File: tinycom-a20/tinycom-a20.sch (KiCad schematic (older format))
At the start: 36 parts, among them P1 CONN_02X08, P2 CONN_02X08, U1 ALLWINNERA10/TFBGA441, U2 H5TQG63BFR/FBGA96, U3 H27UBG8T2A/TSOP48, Y1 Crystal_Small, Y2 Crystal_Small

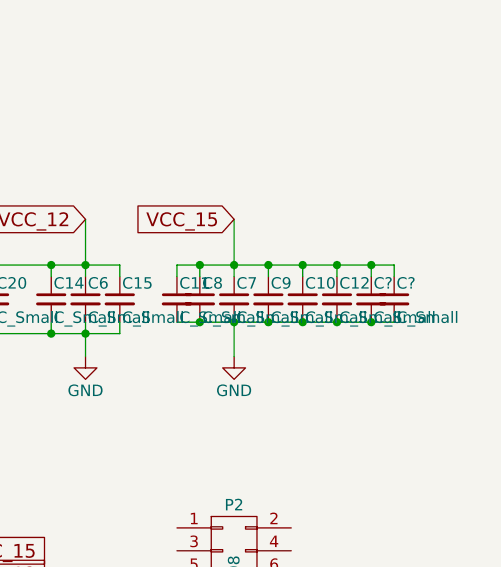
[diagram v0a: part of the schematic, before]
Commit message: add power routes
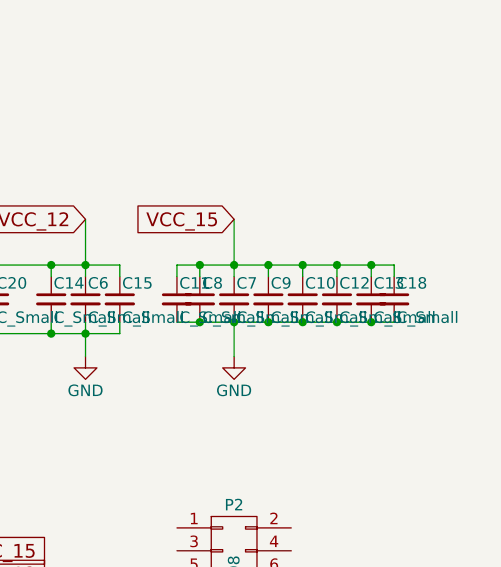
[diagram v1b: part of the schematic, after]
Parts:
- gave numbers to parts that had none: 2
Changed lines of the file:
@@
 $EndComp
 $Comp
-L GND #PWR01
+L GND #PWR21
 U 1 1 563E445F
 P 17800 6150
-F 0 "#PWR01" H 17800 5900 50  0001 C CNN
+F 0 "#PWR21" H 17800 5900 50  0001 C CNN
 F 1 "GND" H 17800 6000 50  0000 C CNN
 F 2 "" H 17800 6150 60  0000 C CNN
@@
 SCK_P
 $Comp
-L GND #PWR02
+L GND #PWR19
 U 1 1 563ECE56
 P 14950 850
-F 0 "#PWR02" H 14950 600 50  0001 C CNN
+F 0 "#PWR19" H 14950 600 50  0001 C CNN
 F 1 "GND" H 14950 700 50  0000 C CNN
 F 2 "" H 14950 850 60  0000 C CNN
@@
 $EndComp
 $Comp
-L GND #PWR03
+L GND #PWR17
 U 1 1 563EDF36
 P 13600 5900
-F 0 "#PWR03" H 13600 5650 50  0001 C CNN
+F 0 "#PWR17" H 13600 5650 50  0001 C CNN
 F 1 "GND" H 13600 5750 50  0000 C CNN
 F 2 "" H 13600 5900 60  0000 C CNN
@@
 $EndComp
 $Comp
-L GND #PWR04
+L GND #PWR18
 U 1 1 563EE398
 P 14350 5150
-F 0 "#PWR04" H 14350 4900 50  0001 C CNN
+F 0 "#PWR18" H 14350 4900 50  0001 C CNN
 F 1 "GND" H 14350 5000 50  0000 C CNN
 F 2 "" H 14350 5150 60  0000 C CNN
@@
 $EndComp
 $Comp
-L GND #PWR05
+L GND #PWR10
 U 1 1 56400687
 P 12400 9950
-F 0 "#PWR05" H 12400 9700 50  0001 C CNN
+F 0 "#PWR10" H 12400 9700 50  0001 C CNN
 F 1 "GND" H 12400 9800 50  0000 C CNN
 F 2 "" H 12400 9950 60  0000 C CNN
@@
 $EndComp
 $Comp
-L GND #PWR06
+L GND #PWR11
 U 1 1 56400704
 P 12650 9950
-F 0 "#PWR06" H 12650 9700 50  0001 C CNN
+F 0 "#PWR11" H 12650 9700 50  0001 C CNN
 F 1 "GND" H 12650 9800 50  0000 C CNN
 F 2 "" H 12650 9950 60  0000 C CNN
@@
 $EndComp
 $Comp
-L GND #PWR07
+L GND #PWR9
 U 1 1 56408532
 P 12150 9250
-F 0 "#PWR07" H 12150 9000 50  0001 C CNN
+F 0 "#PWR9" H 12150 9000 50  0001 C CNN
 F 1 "GND" H 12150 9100 50  0000 C CNN
 F 2 "" H 12150 9250 60  0000 C CNN
@@
 $EndComp
 $Comp
-L GND #PWR08
+L GND #PWR12
 U 1 1 56408573
 P 12700 9300
-F 0 "#PWR08" H 12700 9050 50  0001 C CNN
+F 0 "#PWR12" H 12700 9050 50  0001 C CNN
 F 1 "GND" H 12700 9150 50  0000 C CNN
 F 2 "" H 12700 9300 60  0000 C CNN
@@
 $EndComp
 $Comp
-L GND #PWR09
+L GND #PWR14
 U 1 1 5640D8CA
 P 12750 6950
-F 0 "#PWR09" H 12750 6700 50  0001 C CNN
+F 0 "#PWR14" H 12750 6700 50  0001 C CNN
 F 1 "GND" H 12750 6800 50  0000 C CNN
 F 2 "" H 12750 6950 60  0000 C CNN
@@
 $EndComp
 $Comp
-L GND #PWR010
+L GND #PWR24
 U 1 1 56408FCA
 P 19800 9350
-F 0 "#PWR010" H 19800 9100 50  0001 C CNN
+F 0 "#PWR24" H 19800 9100 50  0001 C CNN
 F 1 "GND" H 19800 9200 50  0000 C CNN
 F 2 "" H 19800 9350 60  0000 C CNN
@@
 UDP2
 $Comp
-L GND #PWR011
+L GND #PWR26
 U 1 1 56411561
 P 20650 10200
-F 0 "#PWR011" H 20650 9950 50  0001 C CNN
+F 0 "#PWR26" H 20650 9950 50  0001 C CNN
 F 1 "GND" H 20650 10050 50  0000 C CNN
 F 2 "" H 20650 10200 60  0000 C CNN
@@
 NoConn ~ 7500 2750
 $Comp
-L GND #PWR012
+L GND #PWR8
 U 1 1 56414A5D
 P 8850 1300
-F 0 "#PWR012" H 8850 1050 50  0001 C CNN
+F 0 "#PWR8" H 8850 1050 50  0001 C CNN
 F 1 "GND" H 8850 1150 50  0000 C CNN
 F 2 "" H 8850 1300 60  0000 C CNN
@@
 VCC_15
 $Comp
-L GND #PWR013
+L GND #PWR1
 U 1 1 56417328
 P 800 9350
-F 0 "#PWR013" H 800 9100 50  0001 C CNN
+F 0 "#PWR1" H 800 9100 50  0001 C CNN
 F 1 "GND" H 800 9200 50  0000 C CNN
 F 2 "" H 800 9350 60  0000 C CNN
@@
 NoConn ~ 1050 13300
 $Comp
-L GND #PWR014
+L GND #PWR3
 U 1 1 56417B02
 P 900 13450
-F 0 "#PWR014" H 900 13200 50  0001 C CNN
+F 0 "#PWR3" H 900 13200 50  0001 C CNN
 F 1 "GND" H 900 13300 50  0000 C CNN
 F 2 "" H 900 13450 60  0000 C CNN
@@
 NoConn ~ 1050 13700
 $Comp
-L GND #PWR015
+L GND #PWR2
 U 1 1 56417F5A
 P 850 13800
-F 0 "#PWR015" H 850 13550 50  0001 C CNN
+F 0 "#PWR2" H 850 13550 50  0001 C CNN
 F 1 "GND" H 850 13650 50  0000 C CNN
 F 2 "" H 850 13800 60  0000 C CNN
@@
 NoConn ~ 5650 11400
 $Comp
-L GND #PWR016
+L GND #PWR6
 U 1 1 56418E41
 P 5850 12050
-F 0 "#PWR016" H 5850 11800 50  0001 C CNN
+F 0 "#PWR6" H 5850 11800 50  0001 C CNN
 F 1 "GND" H 5850 11900 50  0000 C CNN
 F 2 "" H 5850 12050 60  0000 C CNN
@@
 $EndComp
 $Comp
-L GND #PWR017
+L GND #PWR7
 U 1 1 56419222
 P 5900 12300
-F 0 "#PWR017" H 5900 12050 50  0001 C CNN
+F 0 "#PWR7" H 5900 12050 50  0001 C CNN
 F 1 "GND" H 5900 12150 50  0000 C CNN
 F 2 "" H 5900 12300 60  0000 C CNN
@@
 NoConn ~ 11650 14450
 $Comp
-L GND #PWR018
+L GND #PWR16
 U 1 1 5641B53D
 P 12900 9850
-F 0 "#PWR018" H 12900 9600 50  0001 C CNN
+F 0 "#PWR16" H 12900 9600 50  0001 C CNN
 F 1 "GND" H 12900 9700 50  0000 C CNN
 F 2 "" H 12900 9850 60  0000 C CNN
@@
 NoConn ~ 13000 10700
 $Comp
-L GND #PWR019
+L GND #PWR15
 U 1 1 5641BA06
 P 12850 11350
-F 0 "#PWR019" H 12850 11100 50  0001 C CNN
+F 0 "#PWR15" H 12850 11100 50  0001 C CNN
 F 1 "GND" H 12850 11200 50  0000 C CNN
 F 2 "" H 12850 11350 60  0000 C CNN
@@
 NoConn ~ 13000 12600
 $Comp
-L GND #PWR020
+L GND #PWR13
 U 1 1 5641C0BF
 P 12700 12700
-F 0 "#PWR020" H 12700 12450 50  0001 C CNN
+F 0 "#PWR13" H 12700 12450 50  0001 C CNN
 F 1 "GND" H 12700 12550 50  0000 C CNN
 F 2 "" H 12700 12700 60  0000 C CNN
@@
 $EndComp
 $Comp
-L GND #PWR021
+L GND #PWR20
 U 1 1 5641C64B
 P 17750 14500
-F 0 "#PWR021" H 17750 14250 50  0001 C CNN
+F 0 "#PWR20" H 17750 14250 50  0001 C CNN
 F 1 "GND" H 17750 14350 50  0000 C CNN
 F 2 "" H 17750 14500 60  0000 C CNN
@@
 $EndComp
 $Comp
-L GND #PWR022
+L GND #PWR22
 U 1 1 5641CC6D
 P 17800 13850
-F 0 "#PWR022" H 17800 13600 50  0001 C CNN
+F 0 "#PWR22" H 17800 13600 50  0001 C CNN
 F 1 "GND" H 17800 13700 50  0000 C CNN
 F 2 "" H 17800 13850 60  0000 C CNN
@@
 VCC_33
 $Comp
-L GND #PWR023
+L GND #PWR27
 U 1 1 5643044F
 P 20800 13600
-F 0 "#PWR023" H 20800 13350 50  0001 C CNN
+F 0 "#PWR27" H 20800 13350 50  0001 C CNN
 F 1 "GND" H 20800 13450 50  0000 C CNN
 F 2 "" H 20800 13600 60  0000 C CNN
@@
 VCC_33
 $Comp
-L GND #PWR024
+L GND #PWR5
 U 1 1 5643A4FE
 P 5850 10900
-F 0 "#PWR024" H 5850 10650 50  0001 C CNN
+F 0 "#PWR5" H 5850 10650 50  0001 C CNN
 F 1 "GND" H 5850 10750 50  0000 C CNN
 F 2 "" H 5850 10900 60  0000 C CNN
@@
 NoConn ~ 1050 14100
 $Comp
-L GND #PWR025
+L GND #PWR4
 U 1 1 5643BDD7
 P 950 11000
-F 0 "#PWR025" H 950 10750 50  0001 C CNN
+F 0 "#PWR4" H 950 10750 50  0001 C CNN
 F 1 "GND" H 950 10850 50  0000 C CNN
 F 2 "" H 950 11000 60  0000 C CNN
@@
 VCC_33
 $Comp
-L GND #PWR026
+L GND #PWR23
 U 1 1 56440C85
 P 19500 8700
-F 0 "#PWR026" H 19500 8450 50  0001 C CNN
+F 0 "#PWR23" H 19500 8450 50  0001 C CNN
 F 1 "GND" H 19500 8550 50  0000 C CNN
 F 2 "" H 19500 8700 60  0000 C CNN
@@
 $EndComp
 $Comp
-L GND #PWR027
+L GND #PWR25
 U 1 1 56441E51
 P 20300 8700
-F 0 "#PWR027" H 20300 8450 50  0001 C CNN
+F 0 "#PWR25" H 20300 8450 50  0001 C CNN
 F 1 "GND" H 20300 8550 50  0000 C CNN
 F 2 "" H 20300 8700 60  0000 C CNN
@@
 $EndComp
 $Comp
-L GND #PWR028
+L GND #PWR28
 U 1 1 564426D1
 P 20950 8700
-F 0 "#PWR028" H 20950 8450 50  0001 C CNN
+F 0 "#PWR28" H 20950 8450 50  0001 C CNN
 F 1 "GND" H 20950 8550 50  0000 C CNN
 F 2 "" H 20950 8700 60  0000 C CNN
@@
 $EndComp
 $Comp
-L C_Small C?
+L C_Small C13
 U 1 1 5645F6BF
 P 21550 8450
-F 0 "C?" H 21560 8520 50  0000 L CNN
+F 0 "C13" H 21560 8520 50  0000 L CNN
 F 1 "C_Small" H 21560 8370 50  0000 L CNN
 F 2 "Capacitors_SMD:C_0603" H 21550 8450 60  0001 C CNN
@@
 $EndComp
 $Comp
-L C_Small C?
+L C_Small C18
 U 1 1 5645F746
 P 21650 8450
-F 0 "C?" H 21660 8520 50  0000 L CNN
+F 0 "C18" H 21660 8520 50  0000 L CNN
 F 1 "C_Small" H 21660 8370 50  0000 L CNN
 F 2 "Capacitors_SMD:C_0603" H 21650 8450 60  0001 C CNN

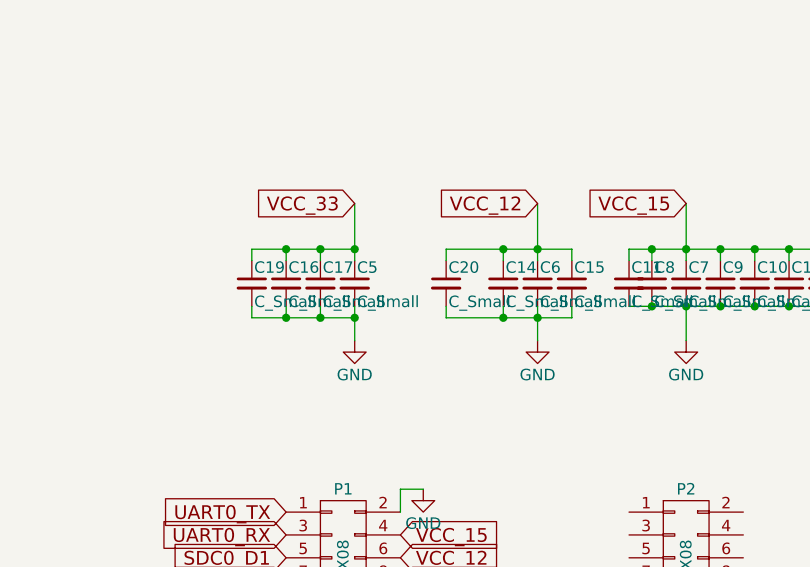
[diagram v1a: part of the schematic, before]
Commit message: fix
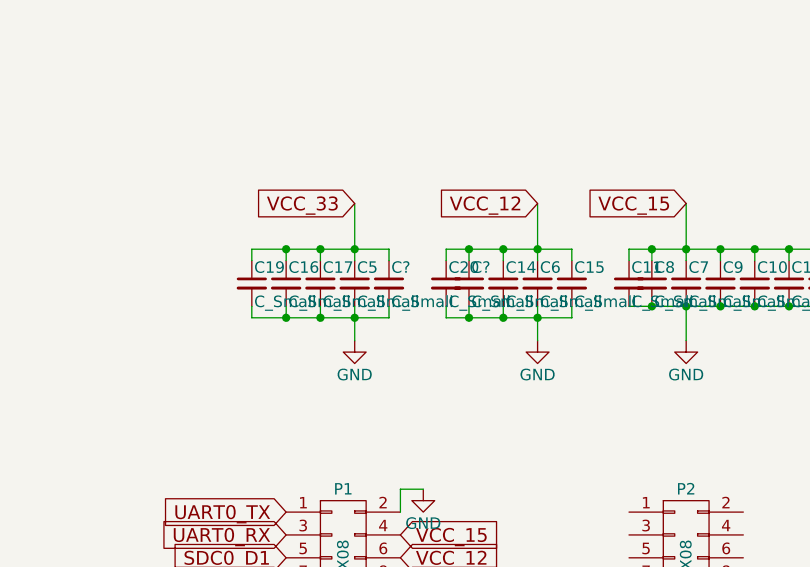
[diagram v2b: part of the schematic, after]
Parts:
- added C? (x2): C_Small, Capacitors_SMD:C_0603, symbol C_Small
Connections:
- net GND: now also C?.2, C?.2
- net VCC_12: now also C?.1
- net VCC_33: now also C?.1
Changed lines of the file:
@@
 	19900 8600 19900 8550
 Wire Wire Line
-	19050 8300 19500 8300
+	19050 8300 19650 8300
 Wire Wire Line
-	19050 8600 19500 8600
+	19050 8600 19650 8600
 Wire Wire Line
 	20700 8550 21650 8550
@@
 Connection ~ 21400 8550
 Connection ~ 21550 8550
+$Comp
+L C_Small C?
+U 1 1 5647248A
+P 20000 8450
+F 0 "C?" H 20010 8520 50  0000 L CNN
+F 1 "C_Small" H 20010 8370 50  0000 L CNN
+F 2 "Capacitors_SMD:C_0603" H 20000 8450 60  0001 C CNN
+F 3 "" H 20000 8450 60  0000 C CNN
+	1    20000 8450
+	1    0    0    -1
+$EndComp
+Wire Wire Line
+	20000 8350 20000 8300
+Connection ~ 20000 8300
+Wire Wire Line
+	20000 8550 20000 8600
+Connection ~ 20000 8600
+$Comp
+L C_Small C?
+U 1 1 56472991
+P 19650 8450
+F 0 "C?" H 19660 8520 50  0000 L CNN
+F 1 "C_Small" H 19660 8370 50  0000 L CNN
+F 2 "Capacitors_SMD:C_0603" H 19650 8450 60  0001 C CNN
+F 3 "" H 19650 8450 60  0000 C CNN
+	1    19650 8450
+	1    0    0    -1
+$EndComp
+Wire Wire Line
+	19650 8300 19650 8350
+Wire Wire Line
+	19650 8600 19650 8550
 $EndSCHEMATC

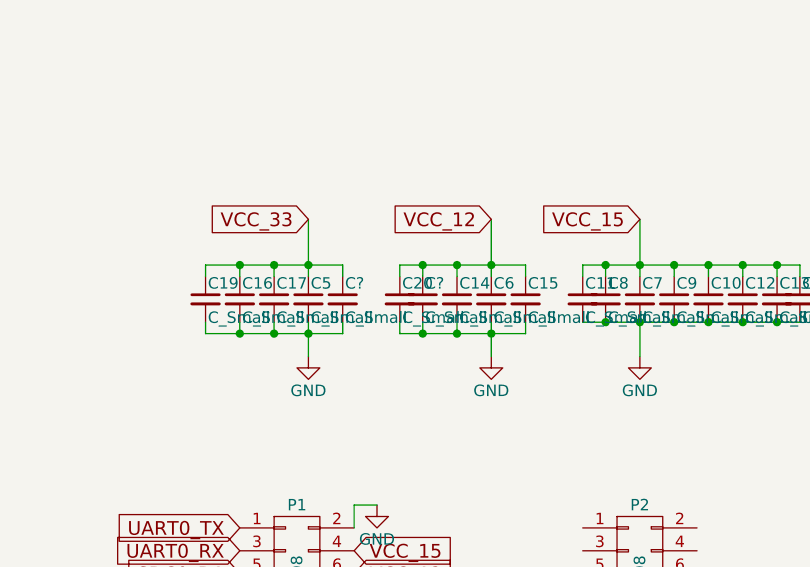
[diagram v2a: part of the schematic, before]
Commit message: readme
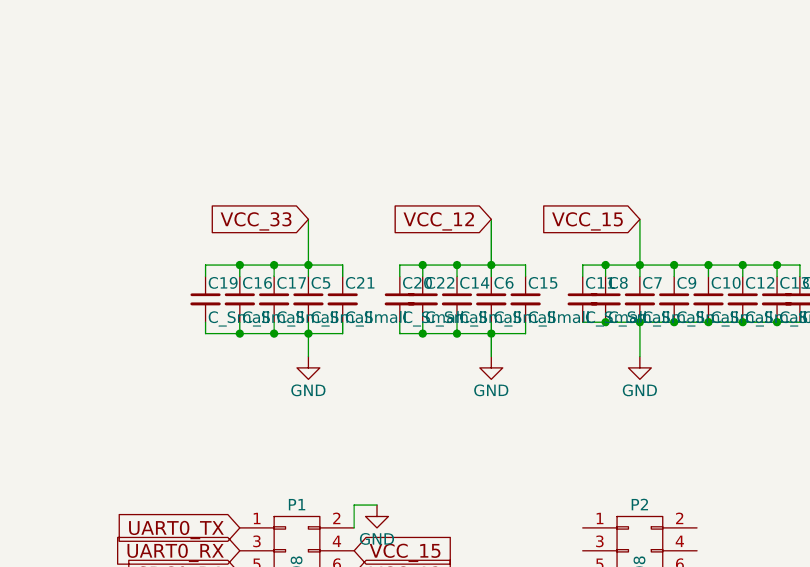
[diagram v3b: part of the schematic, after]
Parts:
- gave numbers to parts that had none: 2
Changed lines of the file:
@@
 $EndComp
 $Comp
-L GND #PWR21
+L GND #PWR01
 U 1 1 563E445F
 P 17800 6150
-F 0 "#PWR21" H 17800 5900 50  0001 C CNN
+F 0 "#PWR01" H 17800 5900 50  0001 C CNN
 F 1 "GND" H 17800 6000 50  0000 C CNN
 F 2 "" H 17800 6150 60  0000 C CNN
@@
 SCK_P
 $Comp
-L GND #PWR19
+L GND #PWR02
 U 1 1 563ECE56
 P 14950 850
-F 0 "#PWR19" H 14950 600 50  0001 C CNN
+F 0 "#PWR02" H 14950 600 50  0001 C CNN
 F 1 "GND" H 14950 700 50  0000 C CNN
 F 2 "" H 14950 850 60  0000 C CNN
@@
 $EndComp
 $Comp
-L GND #PWR17
+L GND #PWR03
 U 1 1 563EDF36
 P 13600 5900
-F 0 "#PWR17" H 13600 5650 50  0001 C CNN
+F 0 "#PWR03" H 13600 5650 50  0001 C CNN
 F 1 "GND" H 13600 5750 50  0000 C CNN
 F 2 "" H 13600 5900 60  0000 C CNN
@@
 $EndComp
 $Comp
-L GND #PWR18
+L GND #PWR04
 U 1 1 563EE398
 P 14350 5150
-F 0 "#PWR18" H 14350 4900 50  0001 C CNN
+F 0 "#PWR04" H 14350 4900 50  0001 C CNN
 F 1 "GND" H 14350 5000 50  0000 C CNN
 F 2 "" H 14350 5150 60  0000 C CNN
@@
 $EndComp
 $Comp
-L GND #PWR10
+L GND #PWR05
 U 1 1 56400687
 P 12400 9950
-F 0 "#PWR10" H 12400 9700 50  0001 C CNN
+F 0 "#PWR05" H 12400 9700 50  0001 C CNN
 F 1 "GND" H 12400 9800 50  0000 C CNN
 F 2 "" H 12400 9950 60  0000 C CNN
@@
 $EndComp
 $Comp
-L GND #PWR11
+L GND #PWR06
 U 1 1 56400704
 P 12650 9950
-F 0 "#PWR11" H 12650 9700 50  0001 C CNN
+F 0 "#PWR06" H 12650 9700 50  0001 C CNN
 F 1 "GND" H 12650 9800 50  0000 C CNN
 F 2 "" H 12650 9950 60  0000 C CNN
@@
 $EndComp
 $Comp
-L GND #PWR9
+L GND #PWR07
 U 1 1 56408532
 P 12150 9250
-F 0 "#PWR9" H 12150 9000 50  0001 C CNN
+F 0 "#PWR07" H 12150 9000 50  0001 C CNN
 F 1 "GND" H 12150 9100 50  0000 C CNN
 F 2 "" H 12150 9250 60  0000 C CNN
@@
 $EndComp
 $Comp
-L GND #PWR12
+L GND #PWR08
 U 1 1 56408573
 P 12700 9300
-F 0 "#PWR12" H 12700 9050 50  0001 C CNN
+F 0 "#PWR08" H 12700 9050 50  0001 C CNN
 F 1 "GND" H 12700 9150 50  0000 C CNN
 F 2 "" H 12700 9300 60  0000 C CNN
@@
 $EndComp
 $Comp
-L GND #PWR14
+L GND #PWR09
 U 1 1 5640D8CA
 P 12750 6950
-F 0 "#PWR14" H 12750 6700 50  0001 C CNN
+F 0 "#PWR09" H 12750 6700 50  0001 C CNN
 F 1 "GND" H 12750 6800 50  0000 C CNN
 F 2 "" H 12750 6950 60  0000 C CNN
@@
 $EndComp
 $Comp
-L GND #PWR24
+L GND #PWR010
 U 1 1 56408FCA
 P 19800 9350
-F 0 "#PWR24" H 19800 9100 50  0001 C CNN
+F 0 "#PWR010" H 19800 9100 50  0001 C CNN
 F 1 "GND" H 19800 9200 50  0000 C CNN
 F 2 "" H 19800 9350 60  0000 C CNN
@@
 UDP2
 $Comp
-L GND #PWR26
+L GND #PWR011
 U 1 1 56411561
 P 20650 10200
-F 0 "#PWR26" H 20650 9950 50  0001 C CNN
+F 0 "#PWR011" H 20650 9950 50  0001 C CNN
 F 1 "GND" H 20650 10050 50  0000 C CNN
 F 2 "" H 20650 10200 60  0000 C CNN
@@
 NoConn ~ 7500 2750
 $Comp
-L GND #PWR8
+L GND #PWR012
 U 1 1 56414A5D
 P 8850 1300
-F 0 "#PWR8" H 8850 1050 50  0001 C CNN
+F 0 "#PWR012" H 8850 1050 50  0001 C CNN
 F 1 "GND" H 8850 1150 50  0000 C CNN
 F 2 "" H 8850 1300 60  0000 C CNN
@@
 VCC_15
 $Comp
-L GND #PWR1
+L GND #PWR013
 U 1 1 56417328
 P 800 9350
-F 0 "#PWR1" H 800 9100 50  0001 C CNN
+F 0 "#PWR013" H 800 9100 50  0001 C CNN
 F 1 "GND" H 800 9200 50  0000 C CNN
 F 2 "" H 800 9350 60  0000 C CNN
@@
 NoConn ~ 1050 13300
 $Comp
-L GND #PWR3
+L GND #PWR014
 U 1 1 56417B02
 P 900 13450
-F 0 "#PWR3" H 900 13200 50  0001 C CNN
+F 0 "#PWR014" H 900 13200 50  0001 C CNN
 F 1 "GND" H 900 13300 50  0000 C CNN
 F 2 "" H 900 13450 60  0000 C CNN
@@
 NoConn ~ 1050 13700
 $Comp
-L GND #PWR2
+L GND #PWR015
 U 1 1 56417F5A
 P 850 13800
-F 0 "#PWR2" H 850 13550 50  0001 C CNN
+F 0 "#PWR015" H 850 13550 50  0001 C CNN
 F 1 "GND" H 850 13650 50  0000 C CNN
 F 2 "" H 850 13800 60  0000 C CNN
@@
 NoConn ~ 5650 11400
 $Comp
-L GND #PWR6
+L GND #PWR016
 U 1 1 56418E41
 P 5850 12050
-F 0 "#PWR6" H 5850 11800 50  0001 C CNN
+F 0 "#PWR016" H 5850 11800 50  0001 C CNN
 F 1 "GND" H 5850 11900 50  0000 C CNN
 F 2 "" H 5850 12050 60  0000 C CNN
@@
 $EndComp
 $Comp
-L GND #PWR7
+L GND #PWR017
 U 1 1 56419222
 P 5900 12300
-F 0 "#PWR7" H 5900 12050 50  0001 C CNN
+F 0 "#PWR017" H 5900 12050 50  0001 C CNN
 F 1 "GND" H 5900 12150 50  0000 C CNN
 F 2 "" H 5900 12300 60  0000 C CNN
@@
 NoConn ~ 11650 14450
 $Comp
-L GND #PWR16
+L GND #PWR018
 U 1 1 5641B53D
 P 12900 9850
-F 0 "#PWR16" H 12900 9600 50  0001 C CNN
+F 0 "#PWR018" H 12900 9600 50  0001 C CNN
 F 1 "GND" H 12900 9700 50  0000 C CNN
 F 2 "" H 12900 9850 60  0000 C CNN
@@
 NoConn ~ 13000 10700
 $Comp
-L GND #PWR15
+L GND #PWR019
 U 1 1 5641BA06
 P 12850 11350
-F 0 "#PWR15" H 12850 11100 50  0001 C CNN
+F 0 "#PWR019" H 12850 11100 50  0001 C CNN
 F 1 "GND" H 12850 11200 50  0000 C CNN
 F 2 "" H 12850 11350 60  0000 C CNN
@@
 NoConn ~ 13000 12600
 $Comp
-L GND #PWR13
+L GND #PWR020
 U 1 1 5641C0BF
 P 12700 12700
-F 0 "#PWR13" H 12700 12450 50  0001 C CNN
+F 0 "#PWR020" H 12700 12450 50  0001 C CNN
 F 1 "GND" H 12700 12550 50  0000 C CNN
 F 2 "" H 12700 12700 60  0000 C CNN
@@
 $EndComp
 $Comp
-L GND #PWR20
+L GND #PWR021
 U 1 1 5641C64B
 P 17750 14500
-F 0 "#PWR20" H 17750 14250 50  0001 C CNN
+F 0 "#PWR021" H 17750 14250 50  0001 C CNN
 F 1 "GND" H 17750 14350 50  0000 C CNN
 F 2 "" H 17750 14500 60  0000 C CNN
@@
 $EndComp
 $Comp
-L GND #PWR22
+L GND #PWR022
 U 1 1 5641CC6D
 P 17800 13850
-F 0 "#PWR22" H 17800 13600 50  0001 C CNN
+F 0 "#PWR022" H 17800 13600 50  0001 C CNN
 F 1 "GND" H 17800 13700 50  0000 C CNN
 F 2 "" H 17800 13850 60  0000 C CNN
@@
 VCC_33
 $Comp
-L GND #PWR27
+L GND #PWR023
 U 1 1 5643044F
 P 20800 13600
-F 0 "#PWR27" H 20800 13350 50  0001 C CNN
+F 0 "#PWR023" H 20800 13350 50  0001 C CNN
 F 1 "GND" H 20800 13450 50  0000 C CNN
 F 2 "" H 20800 13600 60  0000 C CNN
@@
 VCC_33
 $Comp
-L GND #PWR5
+L GND #PWR024
 U 1 1 5643A4FE
 P 5850 10900
-F 0 "#PWR5" H 5850 10650 50  0001 C CNN
+F 0 "#PWR024" H 5850 10650 50  0001 C CNN
 F 1 "GND" H 5850 10750 50  0000 C CNN
 F 2 "" H 5850 10900 60  0000 C CNN
@@
 NoConn ~ 1050 14100
 $Comp
-L GND #PWR4
+L GND #PWR025
 U 1 1 5643BDD7
 P 950 11000
-F 0 "#PWR4" H 950 10750 50  0001 C CNN
+F 0 "#PWR025" H 950 10750 50  0001 C CNN
 F 1 "GND" H 950 10850 50  0000 C CNN
 F 2 "" H 950 11000 60  0000 C CNN
@@
 VCC_33
 $Comp
-L GND #PWR23
+L GND #PWR026
 U 1 1 56440C85
 P 19500 8700
-F 0 "#PWR23" H 19500 8450 50  0001 C CNN
+F 0 "#PWR026" H 19500 8450 50  0001 C CNN
 F 1 "GND" H 19500 8550 50  0000 C CNN
 F 2 "" H 19500 8700 60  0000 C CNN
@@
 $EndComp
 $Comp
-L GND #PWR25
+L GND #PWR027
 U 1 1 56441E51
 P 20300 8700
-F 0 "#PWR25" H 20300 8450 50  0001 C CNN
+F 0 "#PWR027" H 20300 8450 50  0001 C CNN
 F 1 "GND" H 20300 8550 50  0000 C CNN
 F 2 "" H 20300 8700 60  0000 C CNN
@@
 $EndComp
 $Comp
-L GND #PWR28
+L GND #PWR028
 U 1 1 564426D1
 P 20950 8700
-F 0 "#PWR28" H 20950 8450 50  0001 C CNN
+F 0 "#PWR028" H 20950 8450 50  0001 C CNN
 F 1 "GND" H 20950 8550 50  0000 C CNN
 F 2 "" H 20950 8700 60  0000 C CNN
@@
 Connection ~ 21550 8550
 $Comp
-L C_Small C?
+L C_Small C22
 U 1 1 5647248A
 P 20000 8450
-F 0 "C?" H 20010 8520 50  0000 L CNN
+F 0 "C22" H 20010 8520 50  0000 L CNN
 F 1 "C_Small" H 20010 8370 50  0000 L CNN
 F 2 "Capacitors_SMD:C_0603" H 20000 8450 60  0001 C CNN
@@
 Connection ~ 20000 8600
 $Comp
-L C_Small C?
+L C_Small C21
 U 1 1 56472991
 P 19650 8450
-F 0 "C?" H 19660 8520 50  0000 L CNN
+F 0 "C21" H 19660 8520 50  0000 L CNN
 F 1 "C_Small" H 19660 8370 50  0000 L CNN
 F 2 "Capacitors_SMD:C_0603" H 19650 8450 60  0001 C CNN
